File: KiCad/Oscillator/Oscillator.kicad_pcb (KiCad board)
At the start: 2 copper layers, 150 x 130 mm, 173 parts, among them J1 691137710002, J2 691137710003, J3 691137710003, J4 691137710002, J5 691137710002, J6 691137710002, Q1 NPN, Q2 PNP, Q3 NPN, Q4 PNP, Q5 NPN, Q6 NPN, SW1 D6R90F2LFS, SW2 D6R90F2LFS, SW3 D6R90F2LFS, SW4 SW_DPST, U1 CD74HC4051E, U10 TL074, U11 TL074, U2 TL074, U3 TL074, U4 40106, U5 TL074, U6 TL074, U7 TL074, U8 TL074, U9 TL074

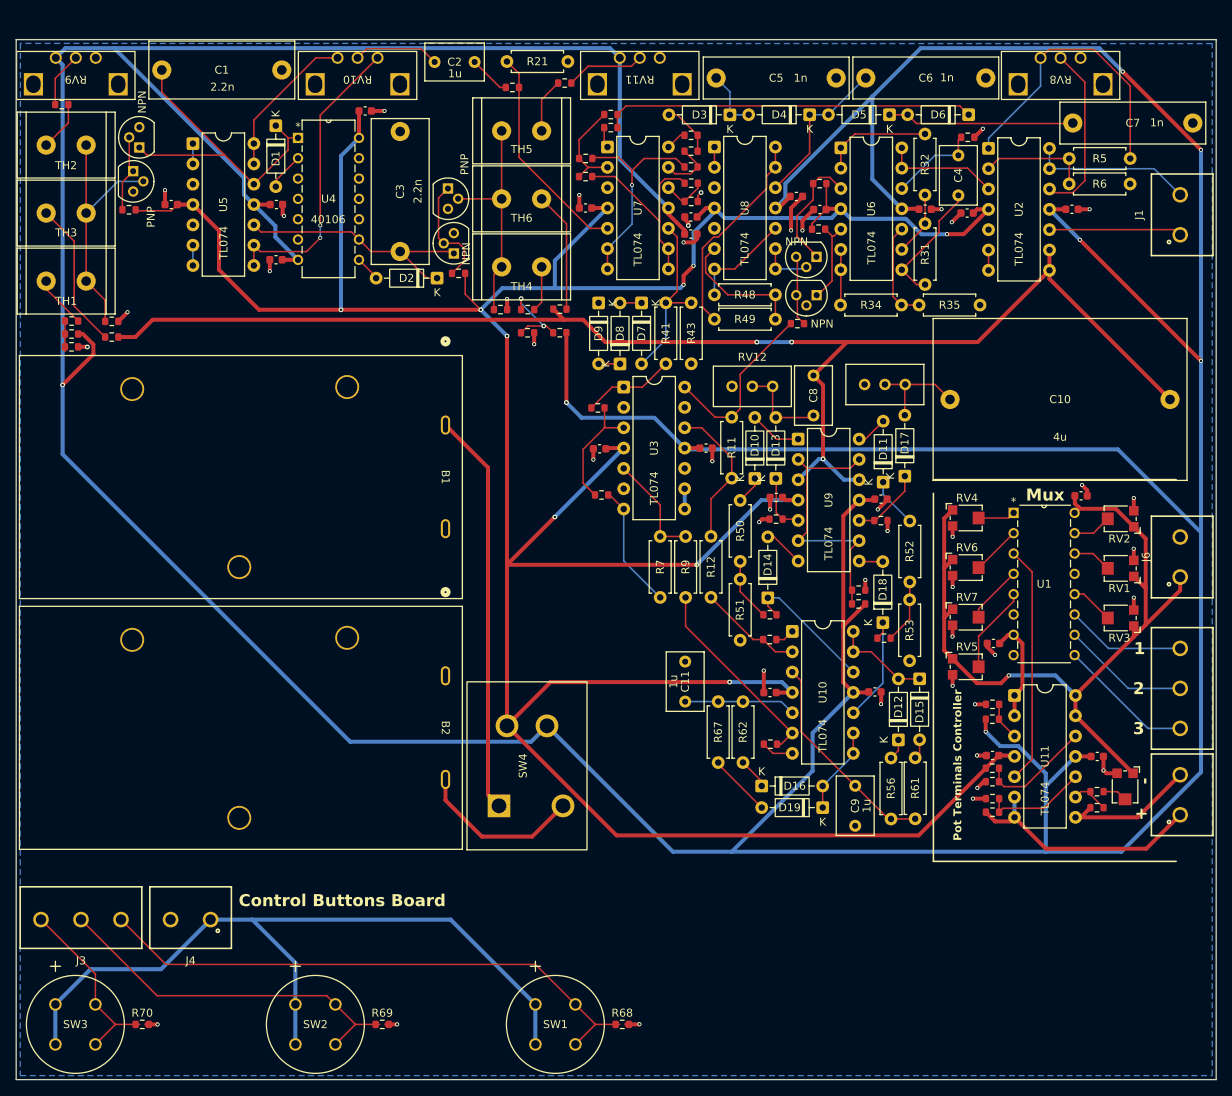
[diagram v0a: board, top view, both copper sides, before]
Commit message: oscillator pcb layout done
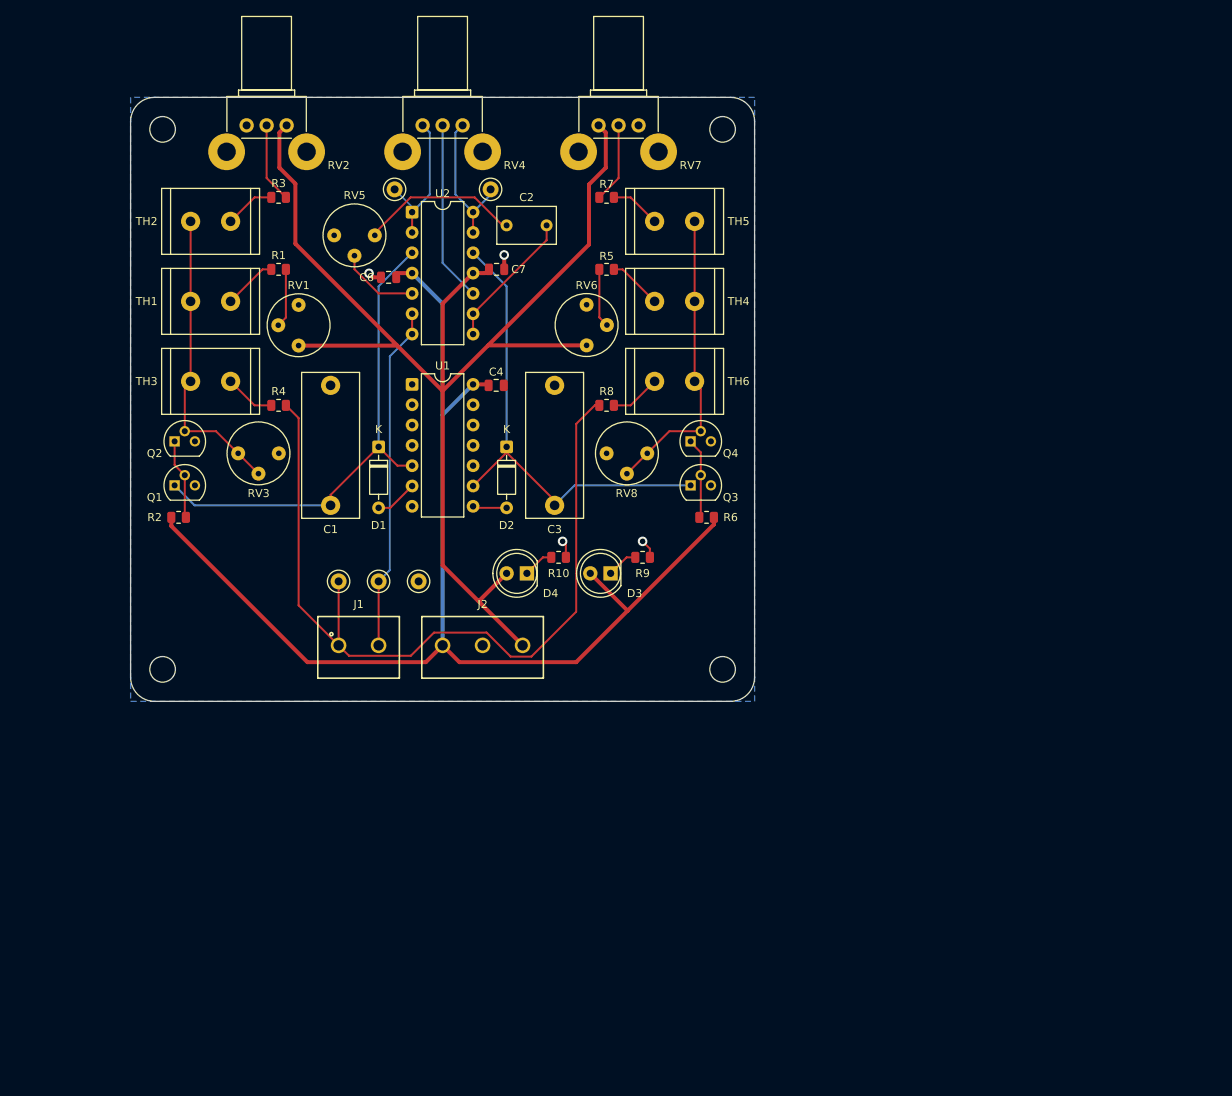
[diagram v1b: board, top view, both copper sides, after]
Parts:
- removed B1, B2: BC9VPC, Battery Holder BC9VPC:BC9VPC_MPD
- removed C10: 4u, Capacitor_THT:C_Rect_L31.5mm_W20.0mm_P27.50mm_MKS4
- removed C11, C8, C9: 1u, Capacitor_THT:C_Rect_L7.2mm_W4.5mm_P5.00mm
- removed C12, C13, C14, C15, C16, C17, C18, C19, C20, C21, C22, C23, C24, C25, C26, C27, C28, C29, C30, C31, C32, C33: 0.1u, Capacitor_SMD:C_0603_1608Metric
- removed C5: 1n, Capacitor_THT:C_Rect_L18.0mm_W5.0mm_P15.00mm_FKS3_FKP3
- removed D10, D11, D12, D13, D14, D15, D16, D17, D18, D19, D5, D6, D7, D8, D9: 1N4148, Diode_THT:D_DO-35_SOD27_P7.62mm_Horizontal
- removed J3: 691137710003, Header 691137710003:691137710003
- removed J4, J5, J6: 691137710002, Header 691137710002:691137710002
- removed Q5, Q6: NPN, Package_TO_SOT_THT:TO-92
- removed R11, R12, R21, R31, R32, R34, R35, R41, R43, R48, R49, R50, R51, R52, R53, R56, R61, R62, R67: R_US, Resistor_THT:R_Axial_DIN0207_L6.3mm_D2.5mm_P7.62mm_Horizontal
- removed R13, R15, R22, R24, R37, R38, R40, R42, R44, R45, R47, R58, R59, R64, R65, R68, R69, R70: 30k, Resistor_SMD:R_0603_1608Metric
- removed R14, R18, R20, R23, R27, R29, R30, R33, R54, R55: 100k, Resistor_SMD:R_0603_1608Metric
- removed R16, R17, R25, R26: 1M, Resistor_SMD:R_0603_1608Metric
- removed R19, R28: 2.4k, Resistor_SMD:R_0603_1608Metric
- removed R36: 10k, Resistor_SMD:R_0603_1608Metric
- removed R39, R46, R60, R66: 1k, Resistor_SMD:R_0603_1608Metric
- removed R71, R74: 15k, Resistor_SMD:R_0603_1608Metric
- removed R72, R73: 12k, Resistor_SMD:R_0603_1608Metric
- removed RV10, RV11, RV9: 100k, Potentiometer 100k PTV09A-2020F-B104:Potentiometer 100k PTV09A-2020F-B104
- removed RV12: 100k, Potentiometer_THT:Potentiometer_Bourns_3296W_Vertical
- removed RV13: 1M, Potentiometer_THT:Potentiometer_Bourns_3296W_Vertical
- removed RV14: 20k, Potentiometer_SMD:Potentiometer_Bourns_TC33X_Vertical
- removed SW1, SW2, SW3: D6R90F2LFS, Switch Push Button D6R90F2LFS:D6R90_CNK
- removed SW4: SW_DPST, DPST Switch RA83231100:DPST Switch RA83231100
- removed U10, U11, U3, U5, U6, U7, U8, U9: TL074, Package_DIP:DIP-14_W7.62mm
- removed U4: 40106, Schmitt Inv. CD40106BE:N14
- added REF**: MountingHole_3.2mm_M3, MountingHole:MountingHole_3.2mm_M3, F.Cu at (114.0, 107.0)
- added REF**: MountingHole_3.2mm_M3, MountingHole:MountingHole_3.2mm_M3, F.Cu at (44.0, 39.5)
- added REF**: MountingHole_3.2mm_M3, MountingHole:MountingHole_3.2mm_M3, F.Cu at (114.0, 39.5)
- added REF**: MountingHole_3.2mm_M3, MountingHole:MountingHole_3.2mm_M3, F.Cu at (44.0, 107.0)
- added TP10: TestPoint_Small, TestPoint:TestPoint_Keystone_5000-5004_Miniature, F.Cu at (73.0, 47.0)
- added TP11: TestPoint_Small, TestPoint:TestPoint_Keystone_5000-5004_Miniature, F.Cu at (76.0, 96.0)
- added TP20: TestPoint_Small, TestPoint:TestPoint_Keystone_5000-5004_Miniature, F.Cu at (85.0, 47.0)
- added TP4: TestPoint_Small, TestPoint:TestPoint_Keystone_5000-5004_Miniature, F.Cu at (66.0, 96.0)
- added TP6: TestPoint_Small, TestPoint:TestPoint_Keystone_5000-5004_Miniature, F.Cu at (71.0, 96.0)
- C4: value 1u -> 0.1u; footprint Capacitor_THT:C_Rect_L7.2mm_W4.5mm_P5.00mm -> Capacitor_SMD:C_0805_2012Metric
- C6, C7: value 1n -> 0.1u; footprint Capacitor_THT:C_Rect_L18.0mm_W5.0mm_P15.00mm_FKS3_FKP3 -> Capacitor_SMD:C_0805_2012Metric
- D3, D4: value 1N4148 -> LED; footprint Diode_THT:D_DO-35_SOD27_P7.62mm_Horizontal -> LED_THT:LED_D5.0mm
- J1: value 691137710002 -> Screw_Terminal_01x02
- J2: value 691137710003 -> Screw_Terminal_01x03
- R1, R4, R8: value 10k -> 100k; footprint Resistor_SMD:R_0603_1608Metric -> Resistor_SMD:R_0805_2012Metric
- R10: value 10k -> 1k; footprint Resistor_SMD:R_0603_1608Metric -> Resistor_SMD:R_0805_2012Metric
- R2, R3: value 10k -> 1M; footprint Resistor_SMD:R_0603_1608Metric -> Resistor_SMD:R_0805_2012Metric
- R5: value R_US -> 100k; footprint Resistor_THT:R_Axial_DIN0207_L6.3mm_D2.5mm_P7.62mm_Horizontal -> Resistor_SMD:R_0805_2012Metric
- R6, R7: value R_US -> 1M; footprint Resistor_THT:R_Axial_DIN0207_L6.3mm_D2.5mm_P7.62mm_Horizontal -> Resistor_SMD:R_0805_2012Metric
- R9: value R_US -> 1k; footprint Resistor_THT:R_Axial_DIN0207_L6.3mm_D2.5mm_P7.62mm_Horizontal -> Resistor_SMD:R_0805_2012Metric
- RV1, RV5, RV6: value 20k -> 100k; footprint Potentiometer_SMD:Potentiometer_Bourns_TC33X_Vertical -> Potentiometer_THT:Potentiometer_Bourns_3339P_Vertical_HandSoldering
- RV2, RV4, RV7: value 20k -> 100k; footprint Potentiometer_SMD:Potentiometer_Bourns_TC33X_Vertical -> Potentiometer_THT:Potentiometer_Bourns_PTV09A-2_Single_Horizontal
- RV3: value 20k -> 5k; footprint Potentiometer_SMD:Potentiometer_Bourns_TC33X_Vertical -> Potentiometer_THT:Potentiometer_Bourns_3339P_Vertical_HandSoldering
- RV8: value 100k -> 5k; footprint Potentiometer 100k PTV09A-2020F-B104:Potentiometer 100k PTV09A-2020F-B104 -> Potentiometer_THT:Potentiometer_Bourns_3339P_Vertical_HandSoldering
- U1: value CD74HC4051E -> 40106; footprint Mux CD74HC4051E:N16 -> Package_DIP:DIP-14_W7.62mm
- moved R3 127.6 mm to (58.5, 48.0)
- moved R1 121.4 mm to (58.5, 57.0)
- moved J1 115.9 mm to (68.5, 104.0), turned to 0 degrees
- moved RV2 115.1 mm to (59.5, 39.0), turned to 90 degrees
- moved R2 108.2 mm to (46.0, 88.0)
- moved RV3 107.1 mm to (58.5, 80.0), turned to 90 degrees
- moved RV1 106.3 mm to (61.0, 66.5), turned to 0 degrees
- moved R4 101.9 mm to (58.5, 74.0), turned to 180 degrees
- moved RV5 91.6 mm to (70.5, 52.8), turned to 90 degrees
- moved U1 89.5 mm to (75.2, 71.4)
- moved C7 88.9 mm to (85.8, 57.0)
- moved J2 87.4 mm to (84.0, 104.0), turned to 0 degrees
- moved RV4 79.9 mm to (81.5, 39.0), turned to 90 degrees
- moved C6 78.7 mm to (72.2, 58.0)
- moved RV7 73.9 mm to (103.5, 39.0), turned to 90 degrees
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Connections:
- C1 pad 1: //Oscillator/Sch Inv In 1 -> /Oscillator/Sch Inv In 1
- C2 pad 1: Net-(C2-Pad1) -> Net-(U2C--)
- C3 pad 1: //Oscillator/Sch Inv In 2 -> /Oscillator/Sch Inv In 2
- C4 pad 1: Net-(C4-Pad1) -> +9V
- C4 pad 2: Net-(U6D-+) -> GND
- C6 pad 1: GND -> +9V
- C6 pad 2: //Filter/Unprocessed Out -> GND
- C7 pad 2: Net-(D5-K) -> -9V
- D1 pad 1: //Oscillator/Sch Inv In 1 -> /Oscillator/Sch Inv In 1
- D1 pad 2: //Oscillator/Sch Inv Out 1 -> /Oscillator/Sch Inv Out 1
- D2 pad 1: //Oscillator/Sch Inv In 2 -> /Oscillator/Sch Inv In 2
- D2 pad 2: //Oscillator/Sch Inv Out 2 -> /Oscillator/Sch Inv Out 2
- D3 pad 2: //Filter/Signal In w. +Offset -> +9V
- D4 pad 1: //Filter/Unprocessed Out -> Net-(D4-K)
- D4 pad 2: Net-(D3-K) -> -9V
- J1 pad 1: //Audio Control -> /Oscillator/Control
- J1 pad 2: //Audio Out -> /Oscillator/Out
- J2 pad 1: /Custom Potentiometer Controls/Trigger 3 -> +9V
- J2 pad 2: /Custom Potentiometer Controls/Trigger 2 -> GND
- J2 pad 3: /Custom Potentiometer Controls/Trigger 1 -> -9V
- Q1 pad 1: //Oscillator/Sch Inv In 1 -> /Oscillator/Sch Inv In 1
- Q2 pad 2: //Oscillator/Core In 1 -> /Oscillator/Processed Control 1
- Q3 pad 1: //Oscillator/Sch Inv In 2 -> /Oscillator/Sch Inv In 2
- Q4 pad 2: //Oscillator/Core In 2 -> /Oscillator/Processed Control 2
- R1 pad 1: /Custom Potentiometer Controls/Pot Voltage Difference -> Net-(R1-Pad1)
- R1 pad 2: Net-(U11C--) -> Net-(R1-Pad2)
- R10 pad 1: Net-(R10-Pad1) -> Net-(D4-K)
- R10 pad 2: Net-(U3A-+) -> GND
- R2 pad 1: /Custom Potentiometer Controls/+Pot -> +9V
- R2 pad 2: Net-(U11C-+) -> Net-(Q1-B)
- R3 pad 1: Net-(U11C--) -> Net-(R3-Pad1)
- R3 pad 2: /Custom Potentiometer Controls/-Pot -> Net-(R3-Pad2)
- R4 pad 1: GND -> /Oscillator/Control
- R4 pad 2: Net-(U11C-+) -> Net-(R4-Pad2)
- R5 pad 1: Net-(U2A--) -> Net-(R5-Pad1)
- R6 pad 1: GND -> +9V
- R6 pad 2: Net-(U2A--) -> Net-(Q3-B)
- R7 pad 1: Net-(U3B-+) -> Net-(R7-Pad1)
- R7 pad 2: Net-(R10-Pad1) -> Net-(R7-Pad2)
- R8 pad 1: Net-(U3A-+) -> /Oscillator/Control
- R8 pad 2: //Filter Control -> Net-(R8-Pad2)
- R9 pad 1: //Envelope Generator/Out Filter -> Net-(D3-K)
- R9 pad 2: Net-(U3B-+) -> GND
- RV1 pad 1: +5V -> -9V
- RV1 pad 2: /Custom Potentiometer Controls/+Pot 1st Partial -> Net-(R1-Pad1)
- RV2 pad 1: +5V -> -9V
- RV2 pad 2: /Custom Potentiometer Controls/+Pot 2nd Partial -> Net-(R3-Pad1)
- RV3 pad 1: +5V -> GND
- RV3 pad 2: /Custom Potentiometer Controls/+Pot 3rd Partial -> /Oscillator/Processed Control 1
- RV3 pad 3: GND -> /Oscillator/Processed Control 1
- RV4 pad 1: +5V -> /Oscillator/Mix In 2
- RV4 pad 2: /Custom Potentiometer Controls/+Pot 4th Partial -> Net-(U2C-+)
- RV4 pad 3: GND -> /Oscillator/Mix In 1
- RV5 pad 1: +5V -> Net-(C2-Pad2)
- RV5 pad 2: /Custom Potentiometer Controls/+Pot 5th Partial -> Net-(U2B-+)
- RV6 pad 1: +5V -> GND
- RV6 pad 2: /Custom Potentiometer Controls/+Pot 6th Partial -> Net-(R5-Pad1)
- RV6 pad 3: GND -> -9V
- RV7 pad 1: +5V -> GND
- RV7 pad 2: /Custom Potentiometer Controls/+Pot 7th Partial -> Net-(R7-Pad1)
- RV7 pad 3: GND -> -9V
- RV8 pad 1: GND -> /Oscillator/Processed Control 2
- RV8 pad 2: Net-(U2D-+) -> /Oscillator/Processed Control 2
- RV8 pad 3: Net-(R5-Pad2) -> GND
- TH1 pad 1: Net-(R14-Pad2) -> Net-(R1-Pad2)
- TH1 pad 2: //Oscillator/Core In 1 -> /Oscillator/Processed Control 1
- TH2 pad 1: Net-(R17-Pad2) -> Net-(R3-Pad2)
- TH2 pad 2: //Oscillator/Core In 1 -> /Oscillator/Processed Control 1
- TH3 pad 1: Net-(R18-Pad2) -> Net-(R4-Pad2)
- TH3 pad 2: //Oscillator/Core In 1 -> /Oscillator/Processed Control 1
- TH4 pad 1: Net-(R23-Pad2) -> Net-(R5-Pad2)
- TH4 pad 2: //Oscillator/Core In 2 -> /Oscillator/Processed Control 2
- TH5 pad 1: Net-(R26-Pad2) -> Net-(R7-Pad2)
- TH5 pad 2: //Oscillator/Core In 2 -> /Oscillator/Processed Control 2
- TH6 pad 1: Net-(R27-Pad2) -> Net-(R8-Pad2)
- TH6 pad 2: //Oscillator/Core In 2 -> /Oscillator/Processed Control 2
- U1 pad 1: /Custom Potentiometer Controls/+Pot 4th Partial -> GND
- U1 pad 10: /Custom Potentiometer Controls/Trigger 2 -> unconnected-(U1-Pad10)
- U1 pad 11: /Custom Potentiometer Controls/Trigger 1 -> GND
- U1 pad 12: /Custom Potentiometer Controls/+Pot 3rd Partial -> unconnected-(U1-Pad12)
- U1 pad 14: /Custom Potentiometer Controls/+Pot 1st Partial -> +9V
- U1 pad 2: /Custom Potentiometer Controls/+Pot 6th Partial -> unconnected-(U1-Pad2)
- U1 pad 3: /Custom Potentiometer Controls/Mux Out -> GND
- U1 pad 4: /Custom Potentiometer Controls/+Pot 7th Partial -> unconnected-(U1-Pad4)
- U1 pad 5: /Custom Potentiometer Controls/+Pot 5th Partial -> /Oscillator/Sch Inv In 1
- U1 pad 6: GND -> /Oscillator/Sch Inv Out 1
- U1 pad 7: -5V -> GND
- U1 pad 8: GND -> /Oscillator/Sch Inv Out 2
- U1 pad 9: /Custom Potentiometer Controls/Trigger 3 -> /Oscillator/Sch Inv In 2
- U2 pad 1: Net-(R5-Pad2) -> /Oscillator/Mix In 1
- U2 pad 10: //Audio Control -> Net-(U2C-+)
- U2 pad 12: Net-(U2D-+) -> /Oscillator/Sch Inv In 2
- U2 pad 13: //Audio Out -> /Oscillator/Mix In 2
- U2 pad 14: //Audio Out -> /Oscillator/Mix In 2
- U2 pad 2: Net-(U2A--) -> /Oscillator/Mix In 1
- U2 pad 3: //Amplifier/Out -> /Oscillator/Sch Inv In 1
- U2 pad 5: GND -> Net-(U2B-+)
- U2 pad 6: /Power/Thaw 2 -> /Oscillator/Out
- U2 pad 7: /Power/Thaw 2 -> /Oscillator/Out
- U2 pad 8: //Buffered Audio Control -> Net-(U2C--)
- U2 pad 9: //Buffered Audio Control -> Net-(U2C--)
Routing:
- net -9V: track 743.4 -> 168.1 mm, vias 7 -> 0
- net +9V: track 418.4 -> 150.3 mm, vias 9 -> 0
- net +5V: track 196.7 -> 0.00 mm, vias 1 -> 0
- net //Buffered Audio Control: track 175.6 -> 0.00 mm, vias 3 -> 0
- net /Oscillator/Control: track 0.00 -> 103.1 mm
- net Net-(J3-Pad1): track 71.3 -> 0.00 mm
- net GND: track 74.3 -> 8.05 mm, vias 44 -> 4
- net /Oscillator/Sch Inv In 1: track 0.00 -> 61.5 mm
- net /Oscillator/Sch Inv In 2: track 0.00 -> 59.8 mm
- net Net-(B1-Pad1): track 50.4 -> 0.00 mm
- net //Filter/Signal In w. -Offset: track 46.4 -> 0.00 mm
- net Net-(J3-Pad2): track 46.3 -> 0.00 mm
- net /Oscillator/Out: track 0.00 -> 43.2 mm
- net //Oscillator/Sch Inv In 1: track 41.1 -> 0.00 mm
- net /Oscillator/Processed Control 2: track 0.00 -> 38.0 mm
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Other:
- board size 150 x 130 mm -> 78 x 75.5 mm
- board text removed: "+"
- board text removed: "-"
- board text removed: "1"
- board text removed: "2"
- board text removed: "3"
- board text removed: "Control Buttons Board"
- board text removed: "Mux"
- board text removed: "Pot Terminals Controller"
